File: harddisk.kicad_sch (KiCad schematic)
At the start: 12 parts, among them IC45 74HCT573, IC46 74HC573, J1 IDC 44-pin IDE

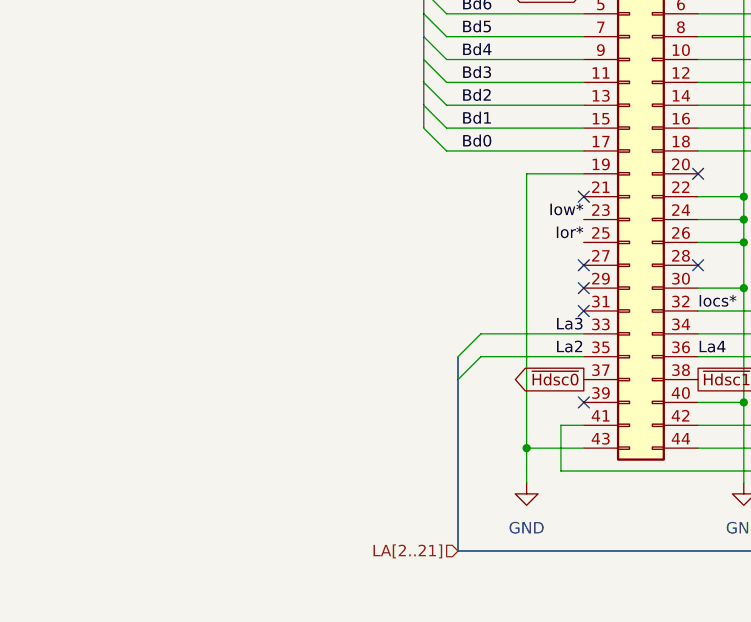
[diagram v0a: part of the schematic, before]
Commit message: fix missing ide signals
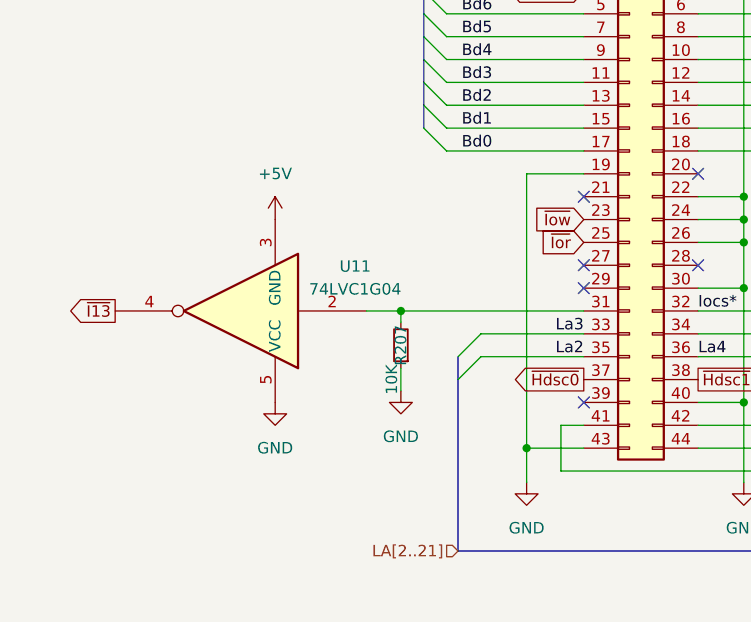
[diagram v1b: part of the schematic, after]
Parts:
- added R207: 10K, Resistor_SMD:R_0805_2012Metric, symbol Device:R_Small
- added U11: 74LVC1G04, Package_TO_SOT_SMD:SOT-353_SC-70-5, symbol 74xGxx:74LVC1G04
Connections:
- net +5V: now also U11.3 (GND)
- net GND: now also R207.1, U11.5 (VCC)
- net at J1.31 (Pin_31): now also R207.2, U11.2
- net Ior* renamed ~{Ior}
- net Iow* renamed ~{Iow}
- new net ~{I13}: U11.4
- no-connect marks 7 -> 6
